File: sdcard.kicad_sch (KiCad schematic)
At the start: 4 parts, among them J12 Micro_SD_Card_Det, U19 RT9742GGJ5

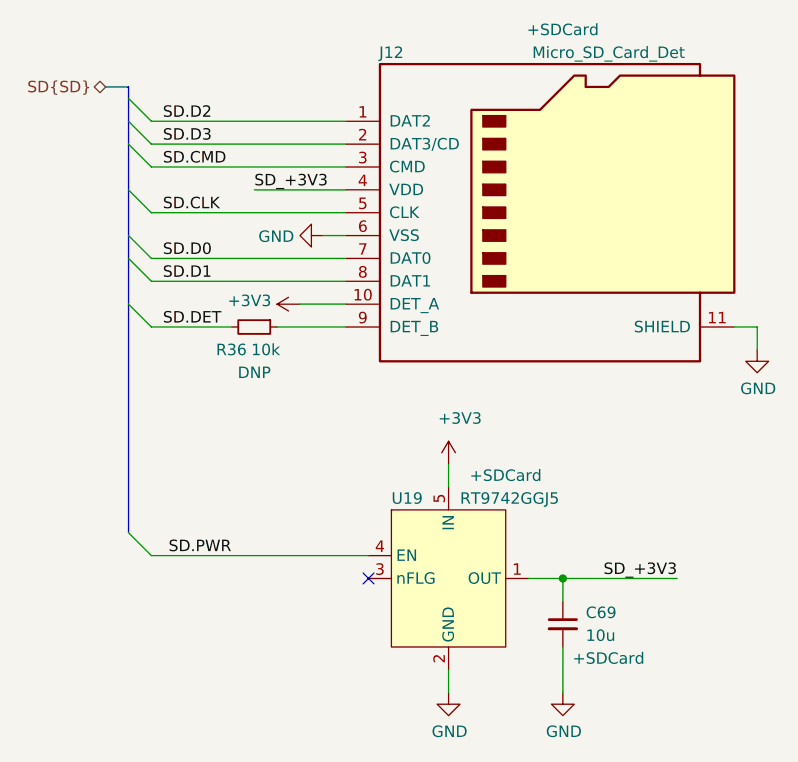
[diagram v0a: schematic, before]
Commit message: [WIP] PCB commit
Signed-off-by: Dominik Sliwa <dominik@sliwa.io>
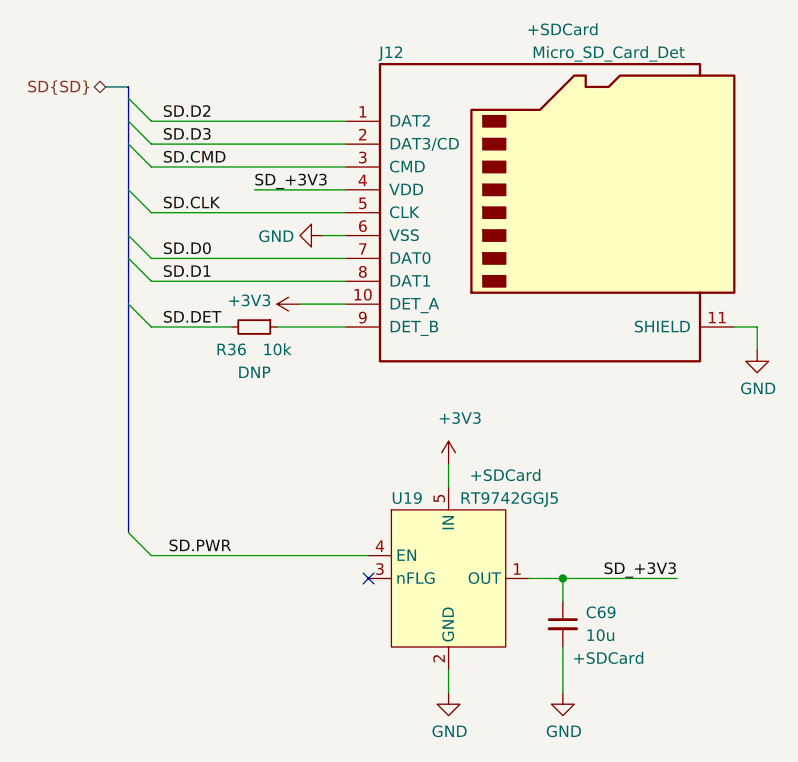
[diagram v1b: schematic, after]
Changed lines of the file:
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@@
     (in_bom yes) (on_board yes)
     (property "Reference" "R36" (id 0) (at 66.675 85.725 90))
-    (property "Value" "10k" (id 1) (at 70.485 85.725 90))
+    (property "Value" "10k" (id 1) (at 71.755 85.725 90))
     (property "Footprint" "Resistor_SMD:R_0402_1005Metric" (id 2) (at 69.215 83.185 0)
       (effects (font (size 1.27 1.27)) hide)
